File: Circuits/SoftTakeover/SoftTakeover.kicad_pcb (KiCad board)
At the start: 2 copper layers, 31.8 x 21.6 mm, 13 parts, among them J1 Conn_01x08_Male, J2 Conn_01x08_Male, J3 Conn_ARM_JTAG_SWD_10, U1 ATSAMD11D14A-M, U2 MCP4728, U3 ADG734

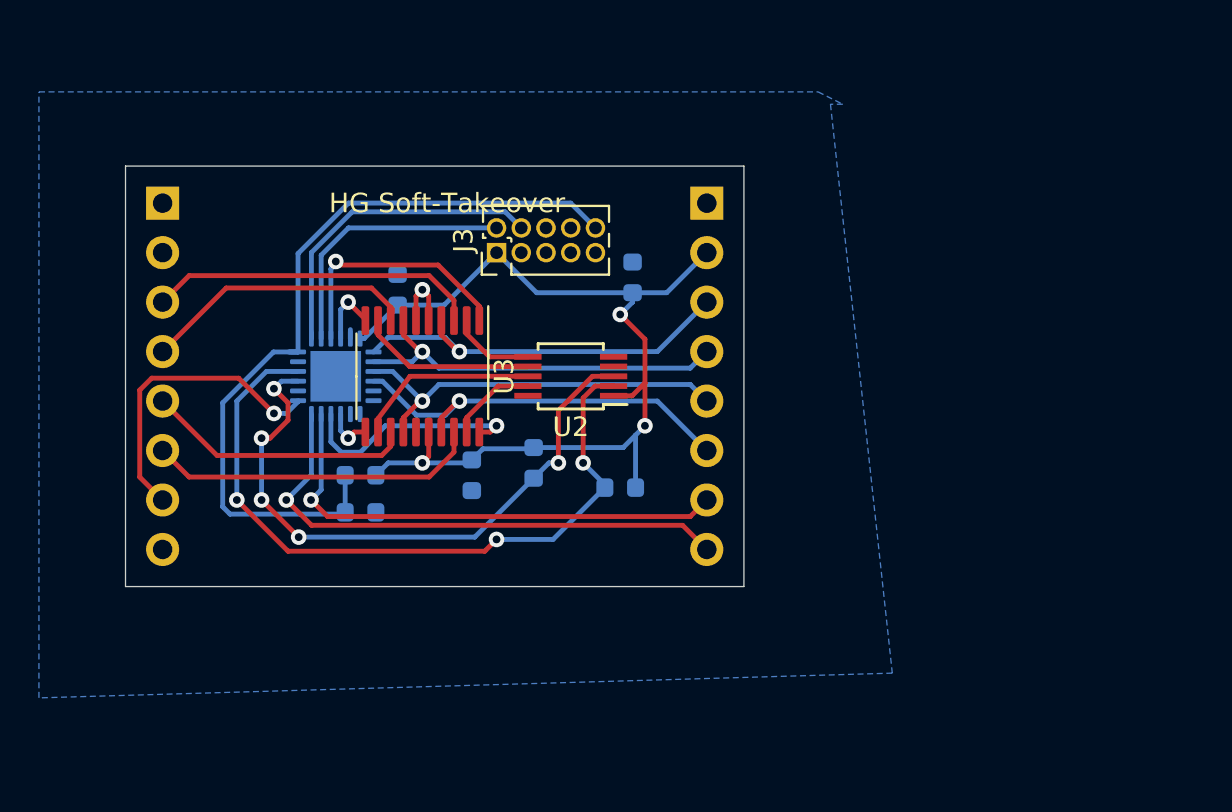
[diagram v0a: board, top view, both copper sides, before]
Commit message: Added various schematics
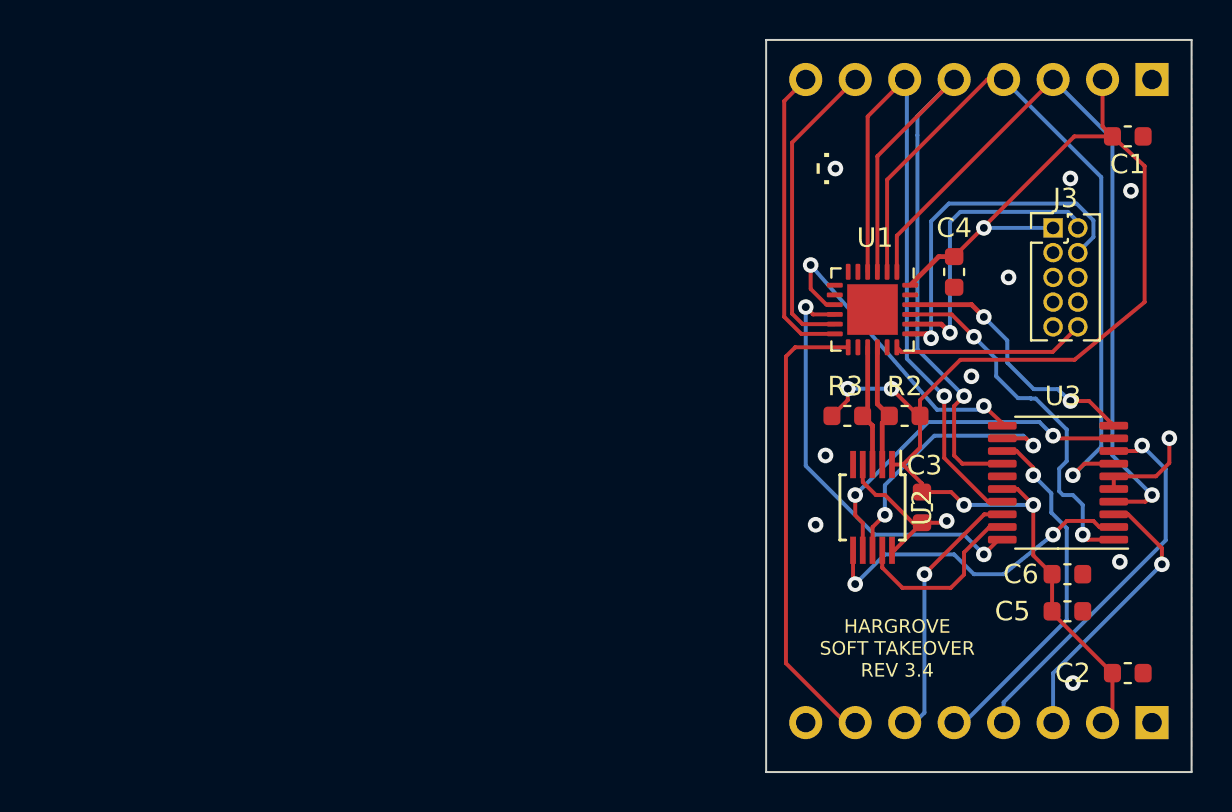
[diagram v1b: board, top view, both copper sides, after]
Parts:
- removed R1: 10k, Resistor_SMD:R_0603_1608Metric
- added C5: 0.1uF, Capacitor_SMD:C_0603_1608Metric, F.Cu at (139.8, 113.7)
- added C6: 1uF, Capacitor_SMD:C_0603_1608Metric, F.Cu at (139.8, 111.8)
- C1, C2, C3, C4: value 100nF -> 0.1uF; moved to F.Cu
- R2, R3, U1: moved to F.Cu
- moved J2 57.4 mm to (144.1, 119.4), turned to 90 degrees
- moved C2 40.3 mm to (142.9, 116.8), turned to 180 degrees
- moved U3 33.1 mm to (139.3, 107.1), turned to 180 degrees
- moved J3 28.6 mm to (139.1, 94.0), turned to 0 degrees
- moved C4 28.6 mm to (134.0, 96.2), turned to 90 degrees
- moved U1 27.8 mm to (129.8, 98.2), turned to 270 degrees
- moved C1 26.4 mm to (142.9, 89.3), turned to 180 degrees
- moved J1 23.7 mm to (144.1, 86.4), turned to 90 degrees
- moved C3 23.2 mm to (132.3, 108.3)
- moved U2 16.9 mm to (129.8, 108.3), turned to 270 degrees
- moved R3 16.3 mm to (128.5, 103.6), turned to 0 degrees
- moved R2 15.1 mm to (131.4, 103.6)
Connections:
- C2 pad 1: RST -> GND
- C2 pad 2: GND -> 3v3
- J3 pad 9: Net-(J3-Pad9) -> GND
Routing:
- net RST: track 41.1 -> 9.92 mm
- net SCL_DAC: track 37.1 -> 6.43 mm, vias 3 -> 0
- net 3v3: track 50.8 -> 76.8 mm, vias 3 -> 5
- net SDA_DAC: track 32.1 -> 6.34 mm, vias 5 -> 0
- net IN_1: track 20.1 -> 38.2 mm
- net IN_0: track 20.8 -> 38.7 mm
- net IN_2: track 20.5 -> 35.4 mm
- net SW_2: track 2.41 -> 16.6 mm, vias 1 -> 2
- net IN_3: track 21.2 -> 34.8 mm
- net DAC_0: track 4.32 -> 17.2 mm, vias 0 -> 2
- net SCL_EXT: track 27.6 -> 15.6 mm, vias 1 -> 0
- net SW_1: track 3.35 -> 13.7 mm, vias 1 -> 2
- net SW_3: track 11.8 -> 22.1 mm, vias 1 -> 2
- net SDA_EXT: track 25.7 -> 16.0 mm, vias 1 -> 0
- net GND: track 3.89 -> 13.3 mm, vias 1 -> 11
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- added copper zone on F.Cu, net GND
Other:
- board size 31.8 x 21.6 mm -> 21.8 x 37.6 mm
- board text added: ".-."
- board text added: "HARGROVE SOFT TAKEOVER REV 3.4"
- board text removed: "HG Soft-Takeover"
